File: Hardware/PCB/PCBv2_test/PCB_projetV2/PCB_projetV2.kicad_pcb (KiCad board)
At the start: 4 copper layers, 63.1 x 41.1 mm, 43 parts, among them J1 Conn_01x02, J10 Conn_02x03_Odd_Even, J11 R-78B5.0-2.0, J12 Conn_01x04, J13 Conn_01x02, J14 Conn_01x02, J2 Conn_01x04, J3 BU33SD5WG-TR, J4 Conn_01x06, J5 Conn_01x03, J6 Conn_01x03, J7 Conn_ST_STDC14, J8 Conn_01x06, J9 Conn_01x06, U1 STM32L552CCTx

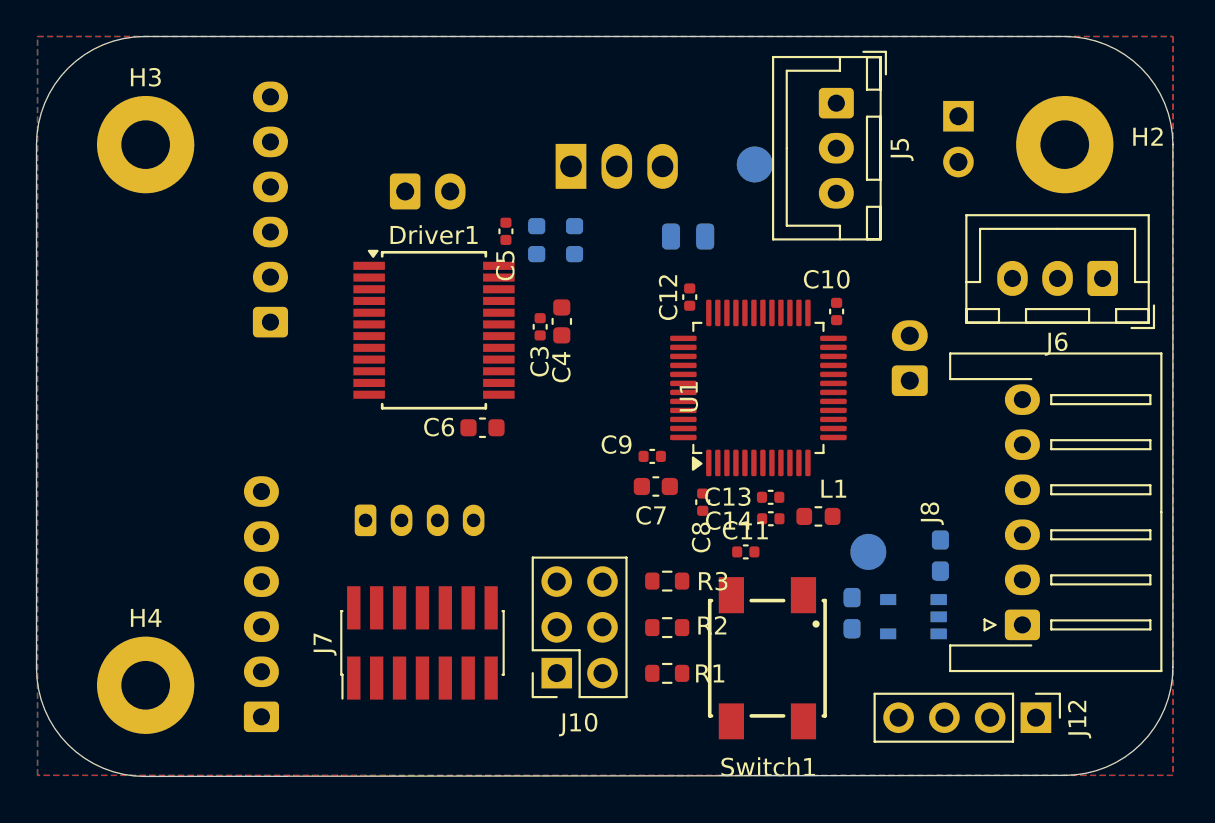
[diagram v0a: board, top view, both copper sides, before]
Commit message: finalisation PCB v2
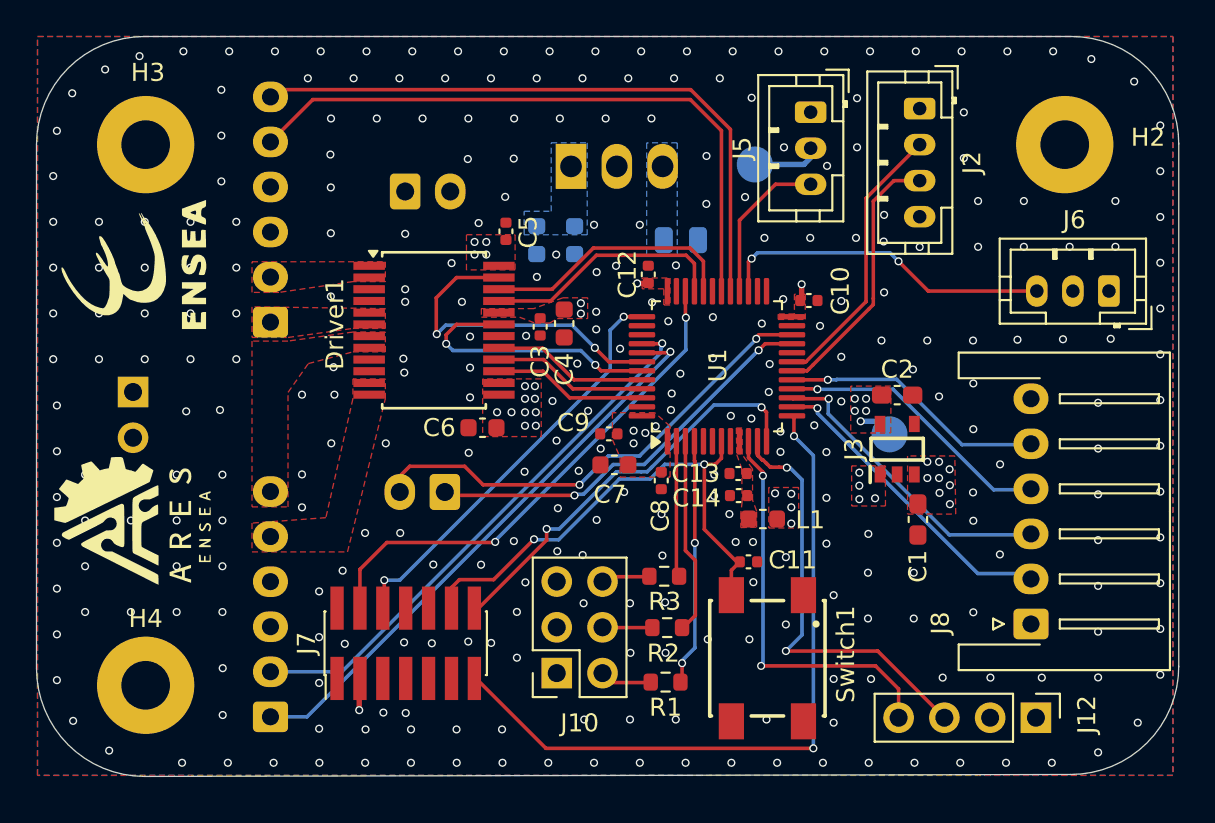
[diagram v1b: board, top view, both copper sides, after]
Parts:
- added G***: LOGO, LogoEnsea:LogoEnsea, F.Cu at (125.7, 86.7)
- added G***: LOGO, LogoAres:logoares, F.Cu at (125.5, 101.0)
- C1, C2, J2, J3: moved to F.Cu
- J5, J6: footprint Connector_JST:JST_XH_B3B-XH-A_1x03_P2.50mm_Vertical -> Connector_JST:JST_PH_B3B-PH-K_1x03_P2.00mm_Vertical
- moved J13 48.3 mm to (125.3, 93.7)
- moved J2 38.3 mm to (168.9, 78.0), turned to -90 degrees
- moved J14 26.5 mm to (142.6, 99.3), turned to 180 degrees
- moved C2 12.4 mm to (167.7, 93.9), turned to 0 degrees
- moved J3 9.34 mm to (167.7, 96.9), turned to 90 degrees
- moved TP2 6.63 mm to (167.3, 96.1), turned to 0 degrees
- moved L1 3.08 mm to (160.2, 100.8)
- moved C9 2.71 mm to (151.7, 96.0)
- moved C12 2.62 mm to (153.9, 87.2)
- moved C7 2.59 mm to (152.0, 97.8)
- moved U1 2.59 mm to (157.7, 92.3)
- moved C8 2.59 mm to (154.6, 98.6)
- moved C1 2.36 mm to (168.8, 100.8), turned to -90 degrees
- moved C13 2.24 mm to (158.9, 98.2)
- moved C14 2.20 mm to (158.9, 99.5)
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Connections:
- net +7.5V renamed +12V
- U1 pad 32: AIN1 -> AIN2
- U1 pad 33: AIN2 -> AIN1
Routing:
- net STLINK_RX: track 0.00 -> 39.4 mm, vias 0 -> 2
- net EncoderA2: track 0.00 -> 35.6 mm
- net EncoderA1: track 0.00 -> 35.6 mm
- net EncoderB2: track 0.00 -> 32.2 mm, vias 0 -> 1
- net EncoderB1: track 0.00 -> 30.7 mm, vias 0 -> 1
- net SWDIO: track 0.00 -> 28.6 mm, vias 0 -> 2
- net NRST: track 0.00 -> 28.4 mm, vias 0 -> 2
- net Rasp_TX: track 0.00 -> 26.9 mm, vias 0 -> 2
- net HC05_TX: track 0.00 -> 24.0 mm, vias 0 -> 2
- net SWCLK: track 0.00 -> 23.2 mm, vias 0 -> 2
- net STLINK_TX: track 0.00 -> 23.0 mm, vias 0 -> 2
- net Rasp_RX: track 0.00 -> 22.8 mm, vias 0 -> 2
- net HC05_RX: track 0.00 -> 22.6 mm, vias 0 -> 2
- net PWM_Servo1: track 0.00 -> 18.7 mm, vias 0 -> 2
- net PWMA: track 0.00 -> 18.4 mm, vias 0 -> 2
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- added copper zone on B.Cu, net +12V
- added copper zone on F.Cu, net +12V
- added copper zone on In2.Cu, net +12V
- added copper zone on F.Cu, net +3.3V
- added copper zone on In2.Cu, net +3.3V
- added copper zone on F.Cu, net +3.3VA
- added copper zone on B.Cu, net +5V
- added copper zone on F.Cu, net +5V
- added copper zone on In2.Cu, net +5V
- added copper zone on F.Cu, net AO1
- added copper zone on F.Cu, net AO2
- added copper zone on F.Cu, net BO1
- added copper zone on F.Cu, net BO2
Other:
- board size 63.1 x 41.1 mm -> 63.4 x 41.1 mm
- board text added: "CAPODAGLI Janus"
- board text added: "Projet 1A"
